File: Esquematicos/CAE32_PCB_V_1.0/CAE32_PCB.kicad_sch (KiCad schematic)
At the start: 2 parts, among them U1 ESP32-S3-WROOM-1, U2 74HC4051

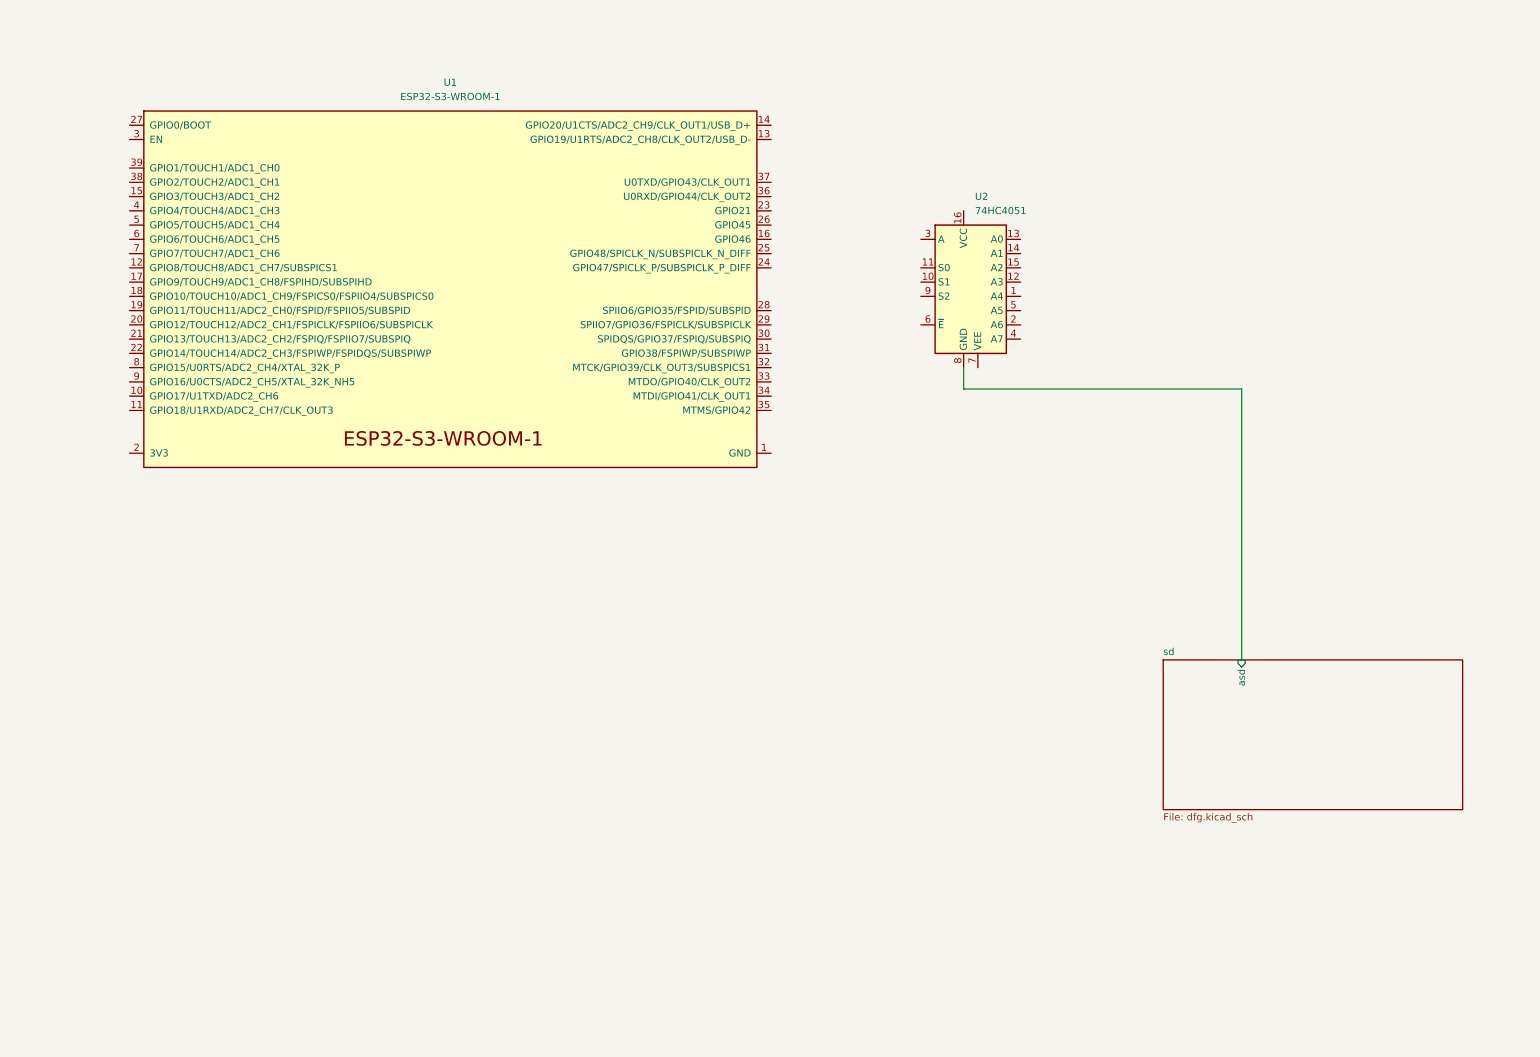
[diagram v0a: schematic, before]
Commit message: Actualización del archivo README
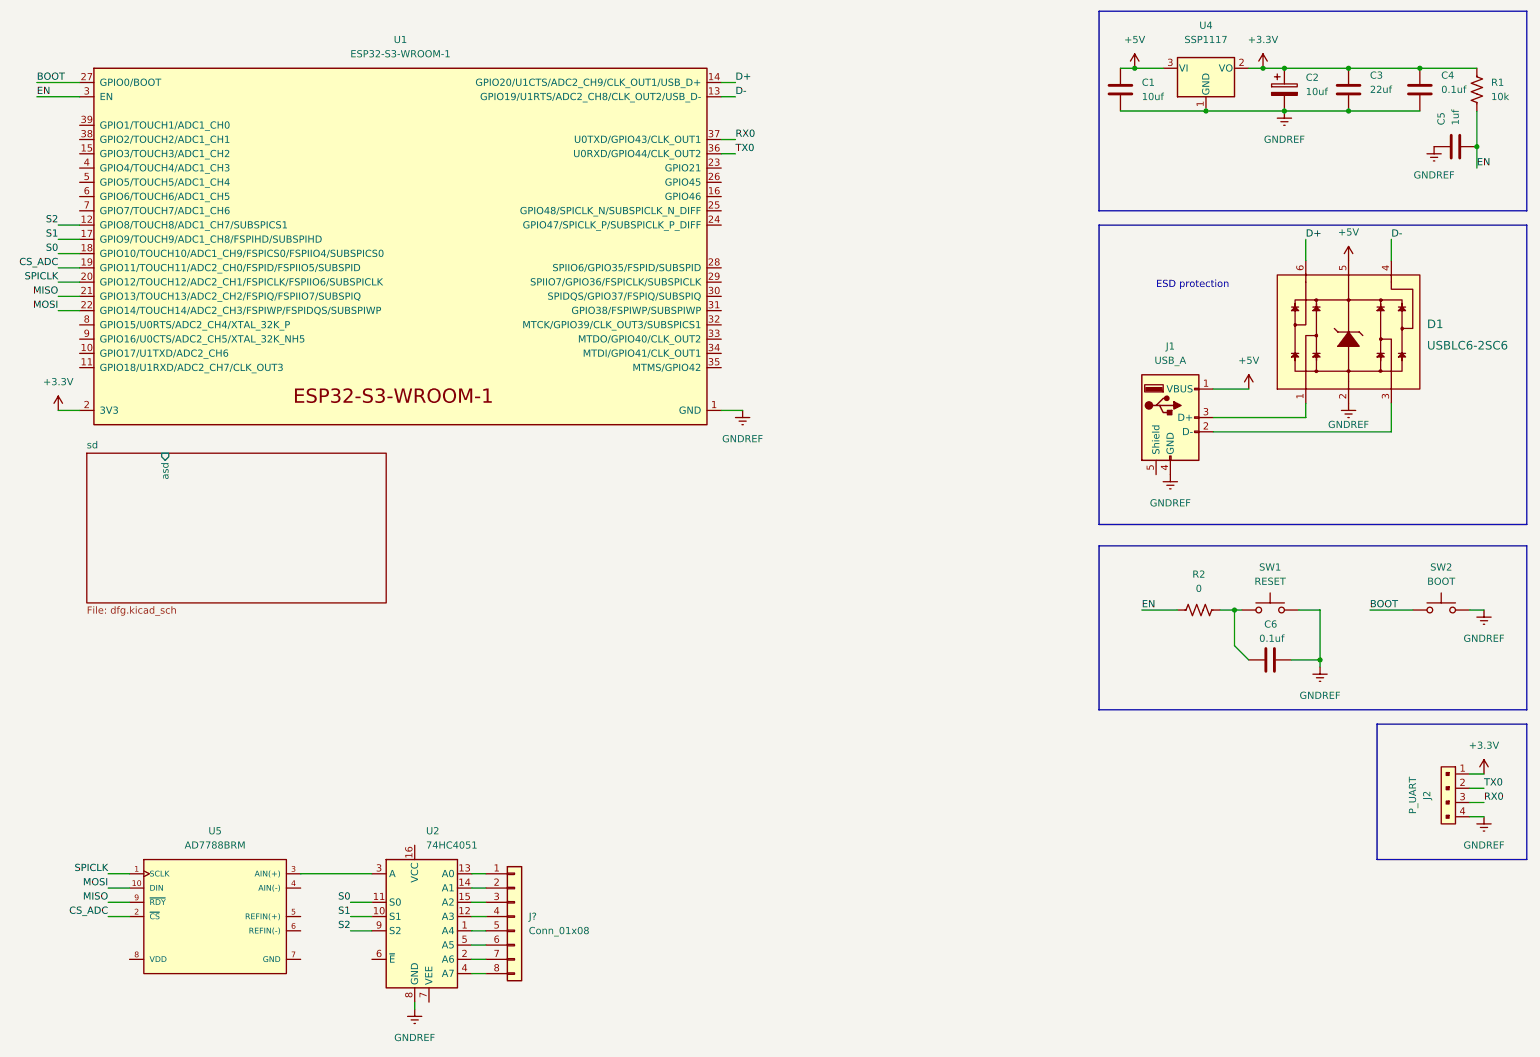
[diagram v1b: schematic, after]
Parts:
- added C1: 10uf, Capacitor_SMD:C_0805_2012Metric, symbol Device:C
- added C2: 10uf, Capacitor_SMD:C_0805_2012Metric, symbol Device:C_Polarized
- added C3: 22uf, Capacitor_SMD:C_0805_2012Metric, symbol Device:C
- added C4, C6: 0.1uf, Capacitor_SMD:C_0805_2012Metric, symbol Device:C
- added C5: 1uf, Capacitor_SMD:C_0805_2012Metric, symbol Device:C
- added D1: USBLC6-2SC6, digikey-footprints:SOT23-6L, symbol dk_TVS-Diodes:USBLC6-2SC6
- added J1: USB_A, Connector_USB:USB_Micro-B_Wuerth_629105150521, symbol Connector:USB_A
- added J2: P_UART, digikey-footprints:PinHeader_1x4_P2.54mm_Drill1.02mm, symbol dk_Rectangular-Connectors-Headers-Male-Pins:0022232041
- added J?: Conn_01x08, symbol Connector_Generic:Conn_01x08
- added R1: 10k, Resistor_SMD:R_0805_2012Metric, symbol Device:R_US
- added R2: 0, Resistor_SMD:R_0805_2012Metric, symbol Device:R_US
- added SW1: RESET, symbol Switch:SW_Push
- added SW2: BOOT, symbol Switch:SW_Push
- added U4: SSP1117, Package_TO_SOT_SMD:SOT-223-3_TabPin2, symbol Regulator_Linear:AP1117-33
- added U5: AD7788BRM, eec:Analog_Devices-AD7788BRM-Level_B, symbol eec:AD7788BRM
- U1: Campo4 (none) -> sdf
- U2: Campo4 (none) -> ffff
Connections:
- net sd/asd: no longer U2.8 (GND)
- net at U2.1 (A4): now also J?.5 (Pin_5)
- net S1: now reaches U2.10 (S1)
- net S1: now also U1.17 (GPIO9/TOUCH9/ADC1_CH8/FSPIHD/SUBSPIHD)
- net S0: now reaches U2.11 (S0)
- net S0: now also U1.18 (GPIO10/TOUCH10/ADC1_CH9/FSPICS0/FSPIIO4/SUBSPICS0)
- net at U2.12 (A3): now also J?.4 (Pin_4)
- net at U2.13 (A0): now also J?.1 (Pin_1)
- net at U2.14 (A1): now also J?.2 (Pin_2)
- net at U2.15 (A2): now also J?.3 (Pin_3)
- net at U2.2 (A6): now also J?.7 (Pin_7)
- net at U2.3 (A): now also U5.3 (AIN(+))
- net at U2.4 (A7): now also J?.8 (Pin_8)
- net at U2.5 (A5): now also J?.6 (Pin_6)
- net S2: now reaches U2.9 (S2)
- net S2: now also U1.12 (GPIO8/TOUCH8/ADC1_CH7/SUBSPICS1)
- net GNDREF: now reaches U1.1 (GND), U1.40 (GND), U1.41 (GND)
- net GNDREF: now also U2.8 (GND), C1.2, C2.2, C3.2, C4.2, C5.1, C6.2, D1.2, J1.4 (GND), J2.4, SW1.2, SW2.2, U4.1 (GND)
- net D-: now reaches U1.13 (GPIO19/U1RTS/ADC2_CH8/CLK_OUT2/USB_D-)
- net D-: now also D1.4
- net D+: now reaches U1.14 (GPIO20/U1CTS/ADC2_CH9/CLK_OUT1/USB_D+)
- net D+: now also D1.6
- net CS_ADC: now reaches U1.19 (GPIO11/TOUCH11/ADC2_CH0/FSPID/FSPIIO5/SUBSPID)
- net CS_ADC: now also U5.2 (~{CS})
- net +3.3V: now reaches U1.2 (3V3)
- net +3.3V: now also C2.1, C3.1, C4.1, J2.1, R1.1, U4.2 (VO)
- net SPICLK: now reaches U1.20 (GPIO12/TOUCH12/ADC2_CH1/FSPICLK/FSPIIO6/SUBSPICLK)
- net SPICLK: now also U5.1 (SCLK)
- net MISO: now reaches U1.21 (GPIO13/TOUCH13/ADC2_CH2/FSPIQ/FSPIIO7/SUBSPIQ)
- net MISO: now also U5.9 (~{RDY})
- net MOSI: now reaches U1.22 (GPIO14/TOUCH14/ADC2_CH3/FSPIWP/FSPIDQS/SUBSPIWP)
- net MOSI: now also U5.10 (DIN)
- net BOOT: now reaches U1.27 (GPIO0/BOOT)
- net BOOT: now also SW2.1
- net EN: now reaches U1.3 (EN)
- net EN: now also C5.2, R1.2, R2.1
- net TX0: now reaches U1.36 (U0RXD/GPIO44/CLK_OUT2)
- net TX0: now also J2.2
- net RX0: now reaches U1.37 (U0TXD/GPIO43/CLK_OUT1)
- net RX0: now also J2.3
- new net: C6.1, R2.2, SW1.1
- new net: D1.3, J1.2 (D-)
- new net: D1.1, J1.3 (D+)
- new net +5V: C1.1, D1.5, J1.1 (VBUS), U4.3 (VI)
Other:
- note added: "ESD protection"
- moved on the sheet: U1, U2
